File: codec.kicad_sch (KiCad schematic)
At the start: 30 parts, among them J10 PJ-327C-4A, J11 PJ-327C-4A, J9 PJ-327C-4A, U15 TAC5111IRGER, U17 LM321, U18 TPA6130A2RTJR

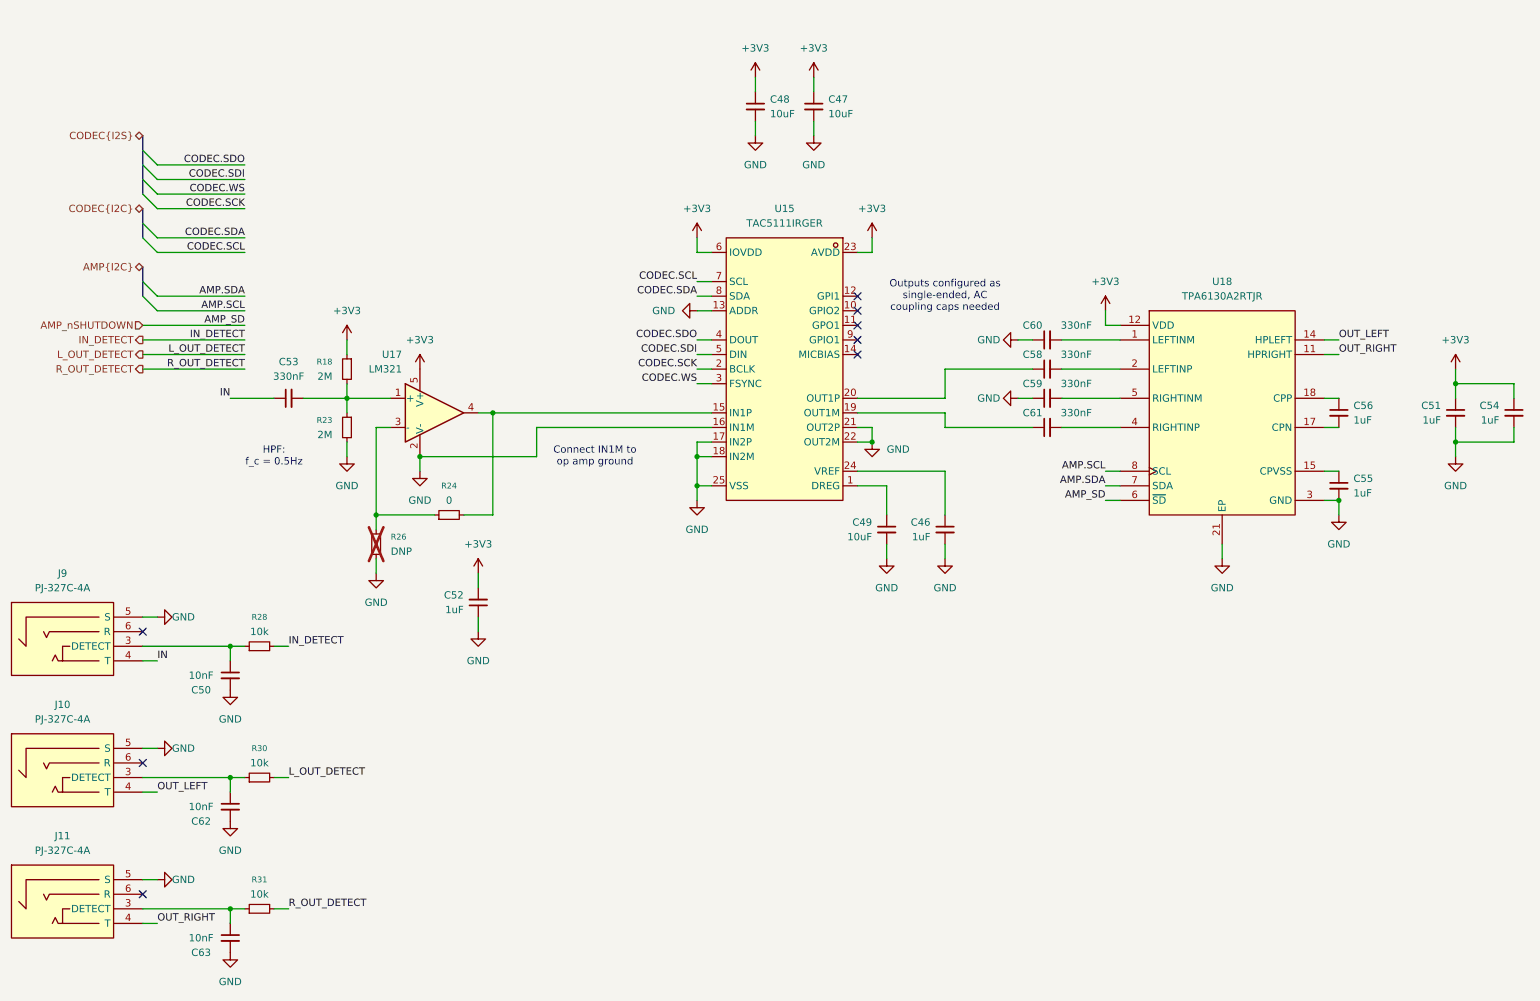
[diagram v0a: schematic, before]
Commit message: OK ACTUALLY ADD JACKS
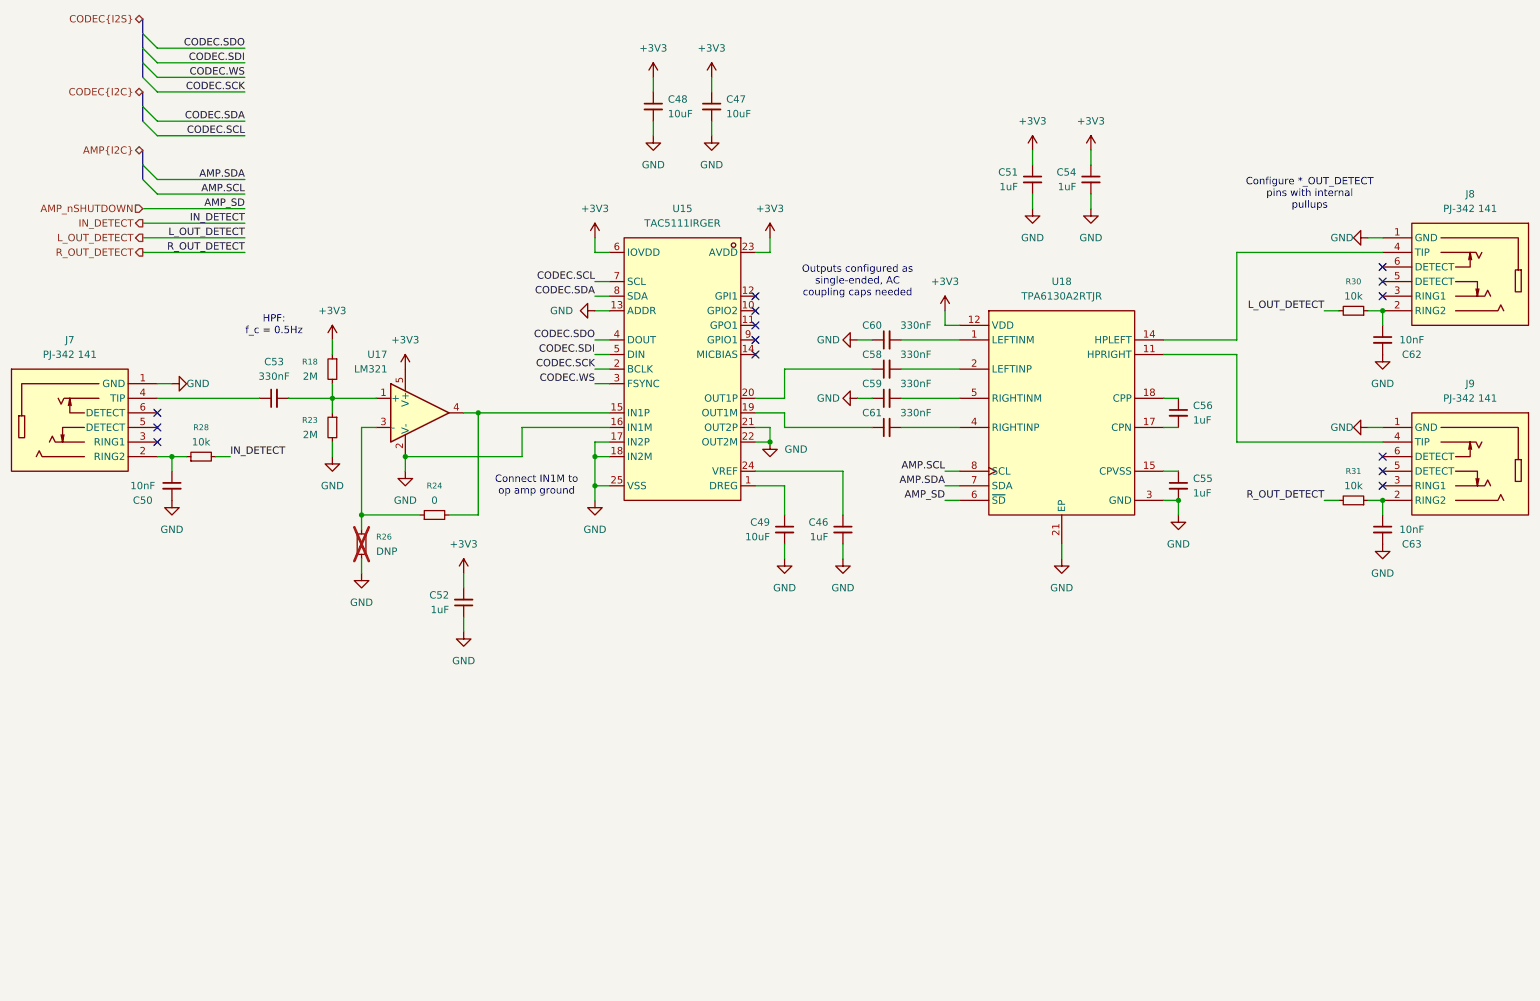
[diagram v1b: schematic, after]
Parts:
- removed J10, J11, J9: PJ-327C-4A, custom:AUDIO-SMD_PJ-327C-4A, symbol custom:PJ-327C-4A
- added J7, J8, J9: PJ-342 141, custom:AUDIO-SMD_PJ-342-141, symbol custom:PJ-342141
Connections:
- net GND: now also J7.1 (GND), J8.1 (GND), J9.1 (GND)
- net at C63.1, R31.1: now also J9.2 (RING2)
- net at C62.1, R30.1: now also J8.2 (RING2)
- net at C50.1, R28.1: now also J7.2 (RING2)
- net IN: no longer names the net of C53.1
- net IN: now also J7.4 (TIP)
- net OUT_LEFT: no longer names the net of U18.14 (HPLEFT)
- net OUT_LEFT: now also J8.4 (TIP)
- net OUT_RIGHT: no longer names the net of U18.11 (HPRIGHT)
- net OUT_RIGHT: now also J9.4 (TIP)
- no-connect marks 8 -> 14
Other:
- note added: "Configure *_OUT_DETECT pins with internal pullups"
- moved on the sheet: C46, C47, C48, C49, C50, C51, C52, C53, C54, C55, C56, C58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
